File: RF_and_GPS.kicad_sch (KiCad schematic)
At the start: 53 parts, among them J22 U.FL-R-SMT-1, J23 U.FL-R-SMT-1, J24 Conn_02x05_Odd_Even, Q1 IRLML2803, SW2 KMR231NG LFS, SW3 KMR231NG LFS, U10 MR25H40MDF, U11 MAX706RESA+, U12 E22-900M30S, U13 S1216V8, U14 EP2W+, U17 RP2040, Y2 ABM8-272-T3

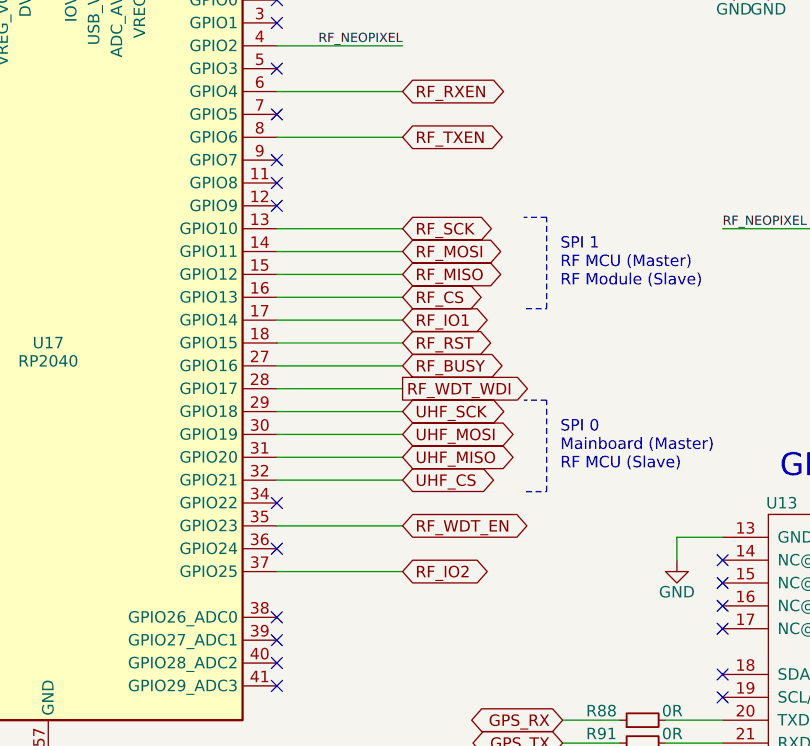
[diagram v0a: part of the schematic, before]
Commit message: Stash
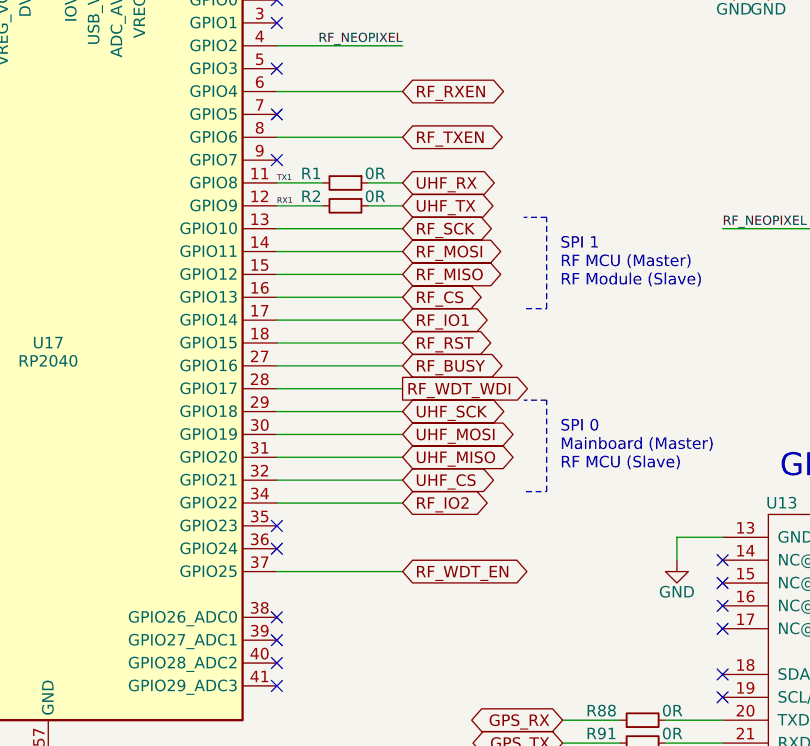
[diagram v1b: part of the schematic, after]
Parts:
- added R1, R2: 0R, Resistor_SMD:R_0603_1608Metric, symbol Device:R_Small
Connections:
- net RF_IO2: now also U17.34 (GPIO22); no longer U17.37 (GPIO25)
- net RF_WDT_EN: now also U17.37 (GPIO25); no longer U17.35 (GPIO23)
- net TX1: now reaches U17.11 (GPIO8)
- net TX1: now also R1.2
- net RX1: now reaches U17.12 (GPIO9)
- net RX1: now also R2.2
- new net UHF_RX: R1.1
- new net UHF_TX: R2.1
- no-connect marks 33 -> 31
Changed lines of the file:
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@@
 	)
 	(no_connect
-		(at 143.51 116.84)
+		(at 143.51 119.38)
 	)
 	(no_connect
@@
 	)
 	(no_connect
-		(at 143.51 83.82)
-	)
-	(no_connect
 		(at 228.6 135.89)
 	)
@@
 	)
 	(no_connect
-		(at 143.51 81.28)
-	)
-	(no_connect
 		(at 143.51 63.5)
 	)
@@
 	(wire
 		(pts
-			(xy 143.51 124.46) (xy 157.48 124.46)
-		)
-		(stroke
-			(width 0)
-			(type default)
-		)
-	)
-	(wire
-		(pts
 			(xy 203.2 86.36) (xy 193.04 86.36)
 		)
@@
 	(wire
 		(pts
+			(xy 143.51 81.28) (xy 148.59 81.28)
+		)
+		(stroke
+			(width 0)
+			(type default)
+		)
+	)
+	(wire
+		(pts
 			(xy 143.51 66.04) (xy 157.48 66.04)
 		)
@@
 	(wire
 		(pts
-			(xy 143.51 119.38) (xy 157.48 119.38)
-		)
-		(stroke
-			(width 0)
-			(type default)
-		)
-	)
-	(wire
-		(pts
 			(xy 67.31 26.67) (xy 67.31 27.94)
 		)
@@
 	(wire
 		(pts
+			(xy 143.51 83.82) (xy 148.59 83.82)
+		)
+		(stroke
+			(width 0)
+			(type default)
+		)
+	)
+	(wire
+		(pts
 			(xy 107.95 34.29) (xy 97.79 34.29)
 		)
@@
 	(wire
 		(pts
+			(xy 153.67 83.82) (xy 157.48 83.82)
+		)
+		(stroke
+			(width 0)
+			(type default)
+		)
+	)
+	(wire
+		(pts
 			(xy 107.95 26.67) (xy 120.65 26.67)
 		)
@@
 	(wire
 		(pts
+			(xy 153.67 81.28) (xy 157.48 81.28)
+		)
+		(stroke
+			(width 0)
+			(type default)
+		)
+	)
+	(wire
+		(pts
 			(xy 250.19 30.48) (xy 250.19 33.02)
 		)
@@
 	(wire
 		(pts
+			(xy 143.51 124.46) (xy 157.48 124.46)
+		)
+		(stroke
+			(width 0)
+			(type default)
+		)
+	)
+	(wire
+		(pts
 			(xy 57.15 34.29) (xy 57.15 35.56)
 		)
@@
 	(wire
 		(pts
+			(xy 143.51 116.84) (xy 157.48 116.84)
+		)
+		(stroke
+			(width 0)
+			(type default)
+		)
+	)
+	(wire
+		(pts
 			(xy 97.79 182.88) (xy 115.57 182.88)
 		)
@@
 		)
 	)
+	(label "RX1"
+		(at 143.51 83.82 0)
+		(fields_autoplaced yes)
+		(effects
+			(font
+				(size 0.635 0.635)
+			)
+			(justify left bottom)
+		)
+	)
 	(label "QSPI_SCK"
 		(at 77.47 93.98 0)
@@
 		)
 	)
+	(label "TX1"
+		(at 143.51 81.28 0)
+		(fields_autoplaced yes)
+		(effects
+			(font
+				(size 0.635 0.635)
+			)
+			(justify left bottom)
+		)
+	)
 	(label "D2+"
 		(at 87.63 68.58 0)
@@
 	(global_label "RF_WDT_EN"
 		(shape bidirectional)
-		(at 157.48 119.38 0)
+		(at 157.48 124.46 0)
 		(fields_autoplaced yes)
 		(effects
@@
 		)
 		(property "Intersheetrefs" "${INTERSHEET_REFS}"
-			(at 171.2258 119.38 0)
+			(at 171.2258 124.46 0)
 			(effects
 				(font
@@
 		)
 	)
-	(global_label "RF_IO2"
+	(global_label "UHF_TX"
 		(shape bidirectional)
-		(at 157.48 124.46 0)
+		(at 157.48 83.82 0)
 		(effects
 			(font
@@
 		)
 		(property "Intersheetrefs" "${INTERSHEET_REFS}"
-			(at 157.48 124.46 0)
+			(at 157.48 83.82 0)
 			(effects
 				(font
 					(size 1.27 1.27)
 				)
-				(justify right)
 				(hide yes)
 			)
@@
 		)
 	)
+	(global_label "RF_IO2"
+		(shape bidirectional)
+		(at 157.48 116.84 0)
+		(effects
+			(font
+				(size 1.27 1.27)
+			)
+			(justify left)
+		)
+		(property "Intersheetrefs" "${INTERSHEET_REFS}"
+			(at 157.48 116.84 0)
+			(effects
+				(font
+					(size 1.27 1.27)
+				)
+				(justify right)
+				(hide yes)
+			)
+		)
+	)
 	(global_label "RF_SWC"
 		(shape bidirectional)
@@
 		)
 	)
+	(global_label "UHF_RX"
+		(shape bidirectional)
+		(at 157.48 81.28 0)
+		(effects
+			(font
+				(size 1.27 1.27)
+			)
+			(justify left)
+		)
+		(property "Intersheetrefs" "${INTERSHEET_REFS}"
+			(at 157.48 81.28 0)
+			(effects
+				(font
+					(size 1.27 1.27)
+				)
+				(hide yes)
+			)
+		)
+	)
 	(global_label "RF_SWC"
 		(shape bidirectional)
@@
 	(symbol
 		(lib_id "Device:R_Small")
+		(at 151.13 81.28 270)
+		(unit 1)
+		(exclude_from_sim no)
+		(in_bom yes)
+		(on_board yes)
+		(dnp no)
+		(property "Reference" "R1"
+			(at 147.32 80.264 90)
+			(effects
+				(font
+					(size 1.27 1.27)
+				)
+			)
+		)
+		(property "Value" "0R"
+			(at 154.432 80.264 90)
+			(effects
+				(font
+					(size 1.27 1.27)
+				)
+			)
+		)
+		(property "Footprint" "Resistor_SMD:R_0603_1608Metric"
+			(at 151.13 81.28 0)
+			(effects
+				(font
+					(size 1.27 1.27)
+				)
+				(hide yes)
+			)
+		)
+		(property "Datasheet" "~"
+			(at 151.13 81.28 0)
+			(effects
+				(font
+					(size 1.27 1.27)
+				)
+				(hide yes)
+			)
+		)
+		(property "Description" "Resistor, small symbol"
+			(at 151.13 81.28 0)
+			(effects
+				(font
+					(size 1.27 1.27)
+				)
+				(hide yes)
+			)
+		)
+		(pin "1"
+		)
+		(pin "2"
+		)
+		(instances
+			(project "Mainboard"
+				(path "/351761a0-c9d1-4ae2-83c5-bde0949aa75f/00000000-0000-0000-0000-00005cec6281"
+					(reference "R1")
+					(unit 1)
+				)
+			)
+		)
+	)
+	(symbol
+		(lib_id "Device:R_Small")
 		(at 85.09 116.84 270)
 		(unit 1)
@@
 	)
 	(symbol
-		(lib_name "Mainboard:KMR231")
 		(lib_id "Mainboard:KMR231")
 		(at 40.64 78.74 0)
@@
 	)
 	(symbol
-		(lib_name "Mainboard:KMR231")
 		(lib_id "Mainboard:KMR231")
 		(at 40.64 60.96 0)
@@
 					(unit 1)
 				)
+			)
+		)
+	)
+	(symbol
+		(lib_id "Device:R_Small")
+		(at 151.13 83.82 270)
+		(unit 1)
+		(exclude_from_sim no)
+		(in_bom yes)
+		(on_board yes)
+		(dnp no)
+		(property "Reference" "R2"
+			(at 147.32 82.804 90)
+			(effects
+				(font
+					(size 1.27 1.27)
+				)
+			)
+		)
+		(property "Value" "0R"
+			(at 154.432 82.804 90)
+			(effects
+				(font
+					(size 1.27 1.27)
+				)
+			)
+		)
+		(property "Footprint" "Resistor_SMD:R_0603_1608Metric"
+			(at 151.13 83.82 0)
+			(effects
+				(font
+					(size 1.27 1.27)
+				)
+				(hide yes)
+			)
+		)
+		(property "Datasheet" "~"
+			(at 151.13 83.82 0)
+			(effects
+				(font
+					(size 1.27 1.27)
+				)
+				(hide yes)
+			)
+		)
+		(property "Description" "Resistor, small symbol"
+			(at 151.13 83.82 0)
+			(effects
+				(font
+					(size 1.27 1.27)
+				)
+				(hide yes)
+			)
+		)
+		(pin "1"
+		)
+		(pin "2"
+		)
+		(instances
+			(project "Mainboard"
+				(path "/351761a0-c9d1-4ae2-83c5-bde0949aa75f/00000000-0000-0000-0000-00005cec6281"
+					(reference "R2")
+					(unit 1)
+				)
